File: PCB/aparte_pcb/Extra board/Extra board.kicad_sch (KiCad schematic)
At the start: 2 parts, among them J1 Conn_01x10_Pin, J2 Conn_01x04_Pin

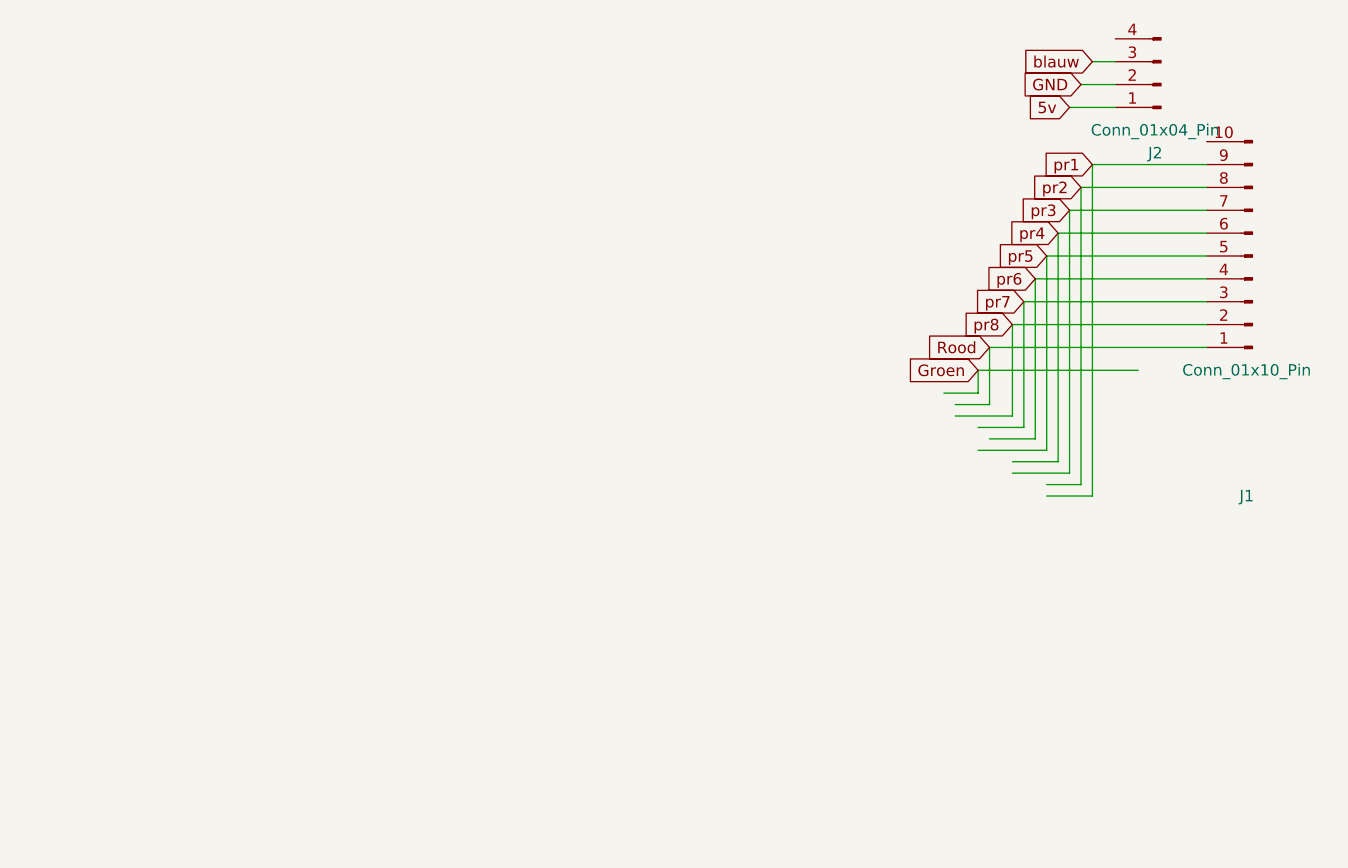
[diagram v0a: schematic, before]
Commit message: Add files via upload
Signed-off-by: Nathan220806 <123752265+Nathan220806@users.noreply.github.com>
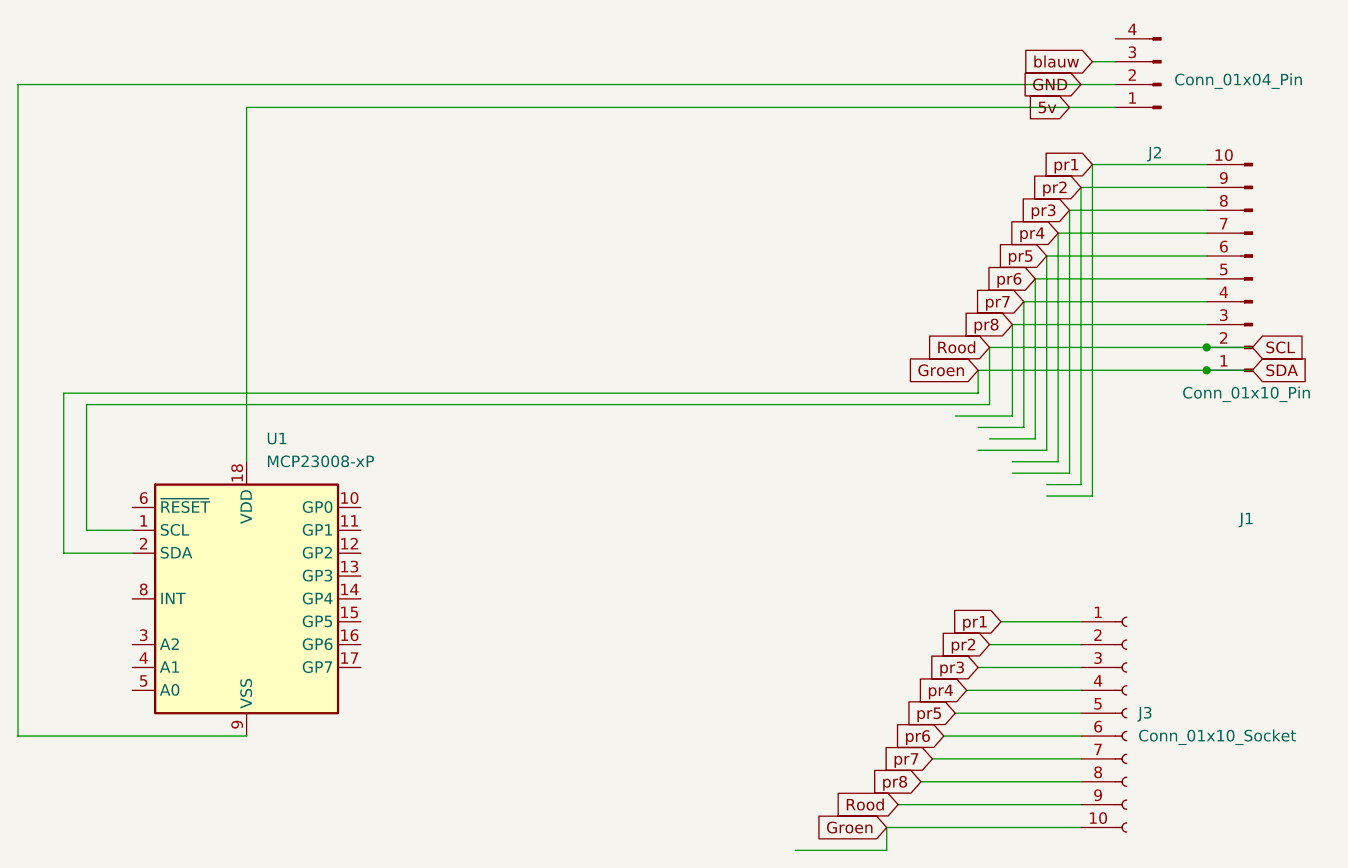
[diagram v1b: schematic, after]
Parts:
- added J3: Conn_01x10_Socket, symbol Connector:Conn_01x10_Socket
- added U1: MCP23008-xP, Package_DIP:DIP-18_W7.62mm, symbol Interface_Expansion:MCP23008-xP
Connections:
- net 5v: now also U1.18 (VDD)
- net GND: now also U1.9 (VSS)
- net Groen: now also J1.1 (Pin_1), J3.10 (Pin_10), U1.2 (SDA)
- net Rood: now also J1.2 (Pin_2), J3.9 (Pin_9), U1.1 (SCL); no longer J1.1 (Pin_1)
- net pr1: now also J1.10 (Pin_10), J3.1 (Pin_1); no longer J1.9 (Pin_9)
- net pr2: now also J1.9 (Pin_9), J3.2 (Pin_2); no longer J1.8 (Pin_8)
- net pr3: now also J1.8 (Pin_8), J3.3 (Pin_3); no longer J1.7 (Pin_7)
- net pr4: now also J1.7 (Pin_7), J3.4 (Pin_4); no longer J1.6 (Pin_6)
- net pr5: now also J1.6 (Pin_6), J3.5 (Pin_5); no longer J1.5 (Pin_5)
- net pr6: now also J1.5 (Pin_5), J3.6 (Pin_6); no longer J1.4 (Pin_4)
- net pr7: now also J1.4 (Pin_4), J3.7 (Pin_7); no longer J1.3 (Pin_3)
- net pr8: now also J1.3 (Pin_3), J3.8 (Pin_8); no longer J1.2 (Pin_2)
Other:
- moved on the sheet: J1
